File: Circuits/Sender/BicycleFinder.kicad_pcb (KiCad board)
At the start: 2 copper layers, 64.1 x 40.1 mm, 11 parts, among them CN1 WRITER, SW1 SW_PUSH, U1 LITE_LITE, U2 HN2S01FU

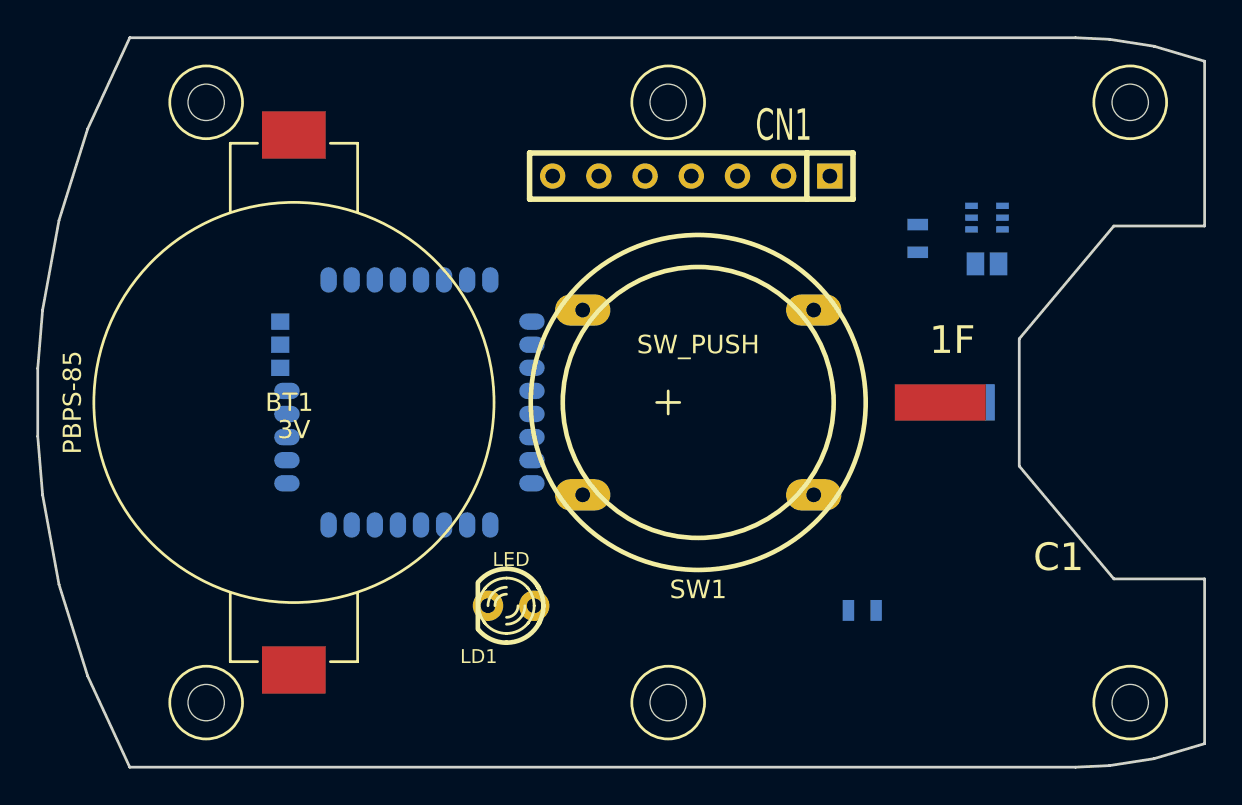
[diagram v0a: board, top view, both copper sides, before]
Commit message: Reviewed parts layout.
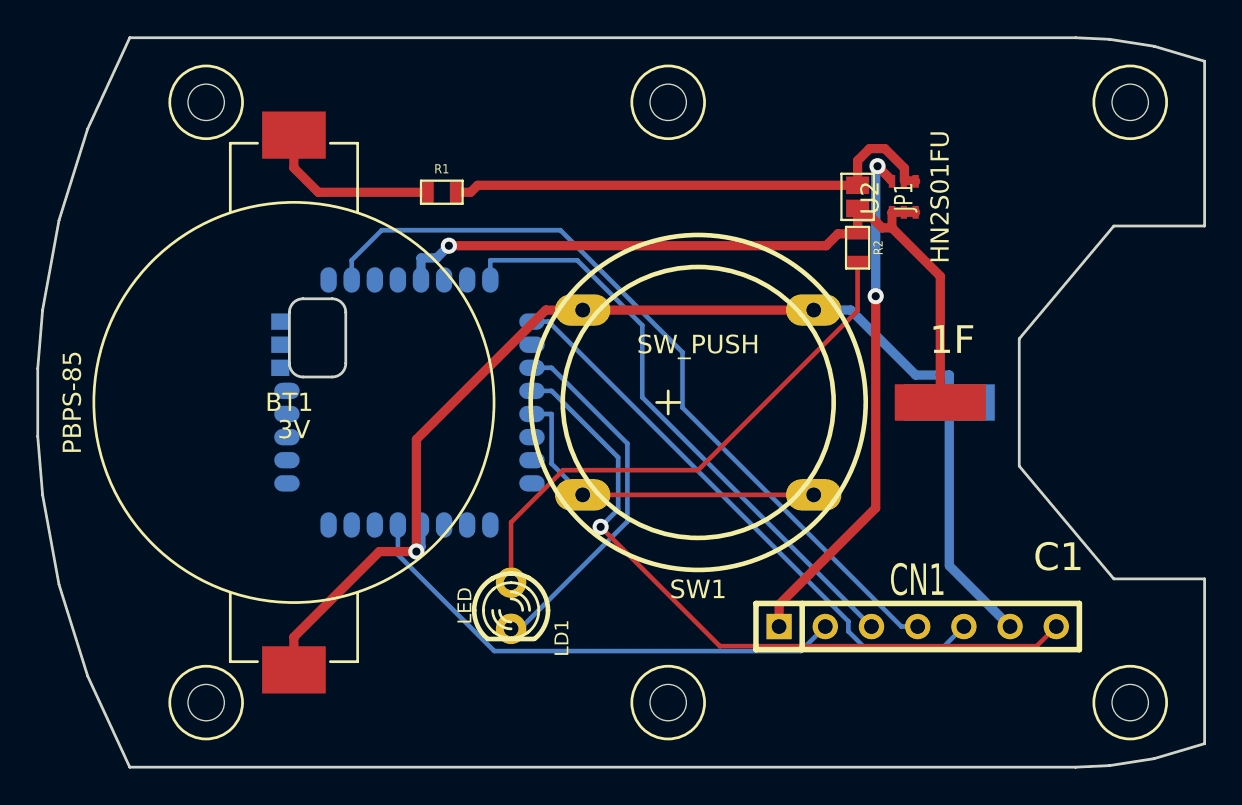
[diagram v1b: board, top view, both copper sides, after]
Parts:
- JP1, R1, R2, U2: moved to F.Cu
- U1: footprint TWE-001L-SMD-noNTH -> TWE-001L-SMD
- moved CN1 27.7 mm to (214.6, 148.8), turned to 0 degrees
- moved R1 26.3 mm to (188.5, 125.0), turned to 0 degrees
- moved R2 19.9 mm to (211.3, 128.0), turned to 90 degrees
- moved JP1 8.01 mm to (211.3, 125.2), turned to 180 degrees
- moved U2 4.71 mm to (213.9, 125.2), turned to 90 degrees
- turned LD1 to 270 degrees
- turned U1 to 270 degrees
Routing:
- net GND: track 0.00 -> 67.2 mm, vias 0 -> 1
- net /PRG: track 0.00 -> 43.7 mm
- net /Vcc: track 0.00 -> 42.1 mm, vias 0 -> 1
- net /M1: track 0.00 -> 38.7 mm, vias 0 -> 1
- net /RX: track 0.00 -> 32.7 mm
- net /TX: track 0.00 -> 31.9 mm
- net /LED: track 0.00 -> 29.9 mm
- net /DC3V: track 0.00 -> 28.7 mm, vias 0 -> 2
- net /CHG: track 0.00 -> 28.3 mm
- net /RST: track 0.00 -> 27.9 mm
- net /DO4: track 0.00 -> 20.1 mm
- net /DI1: track 0.00 -> 18.9 mm
- net /3V: track 0.00 -> 9.73 mm
